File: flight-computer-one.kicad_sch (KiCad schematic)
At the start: 6 parts, among them J3 Screw_Terminal_01x08, J4 Screw_Terminal_01x08

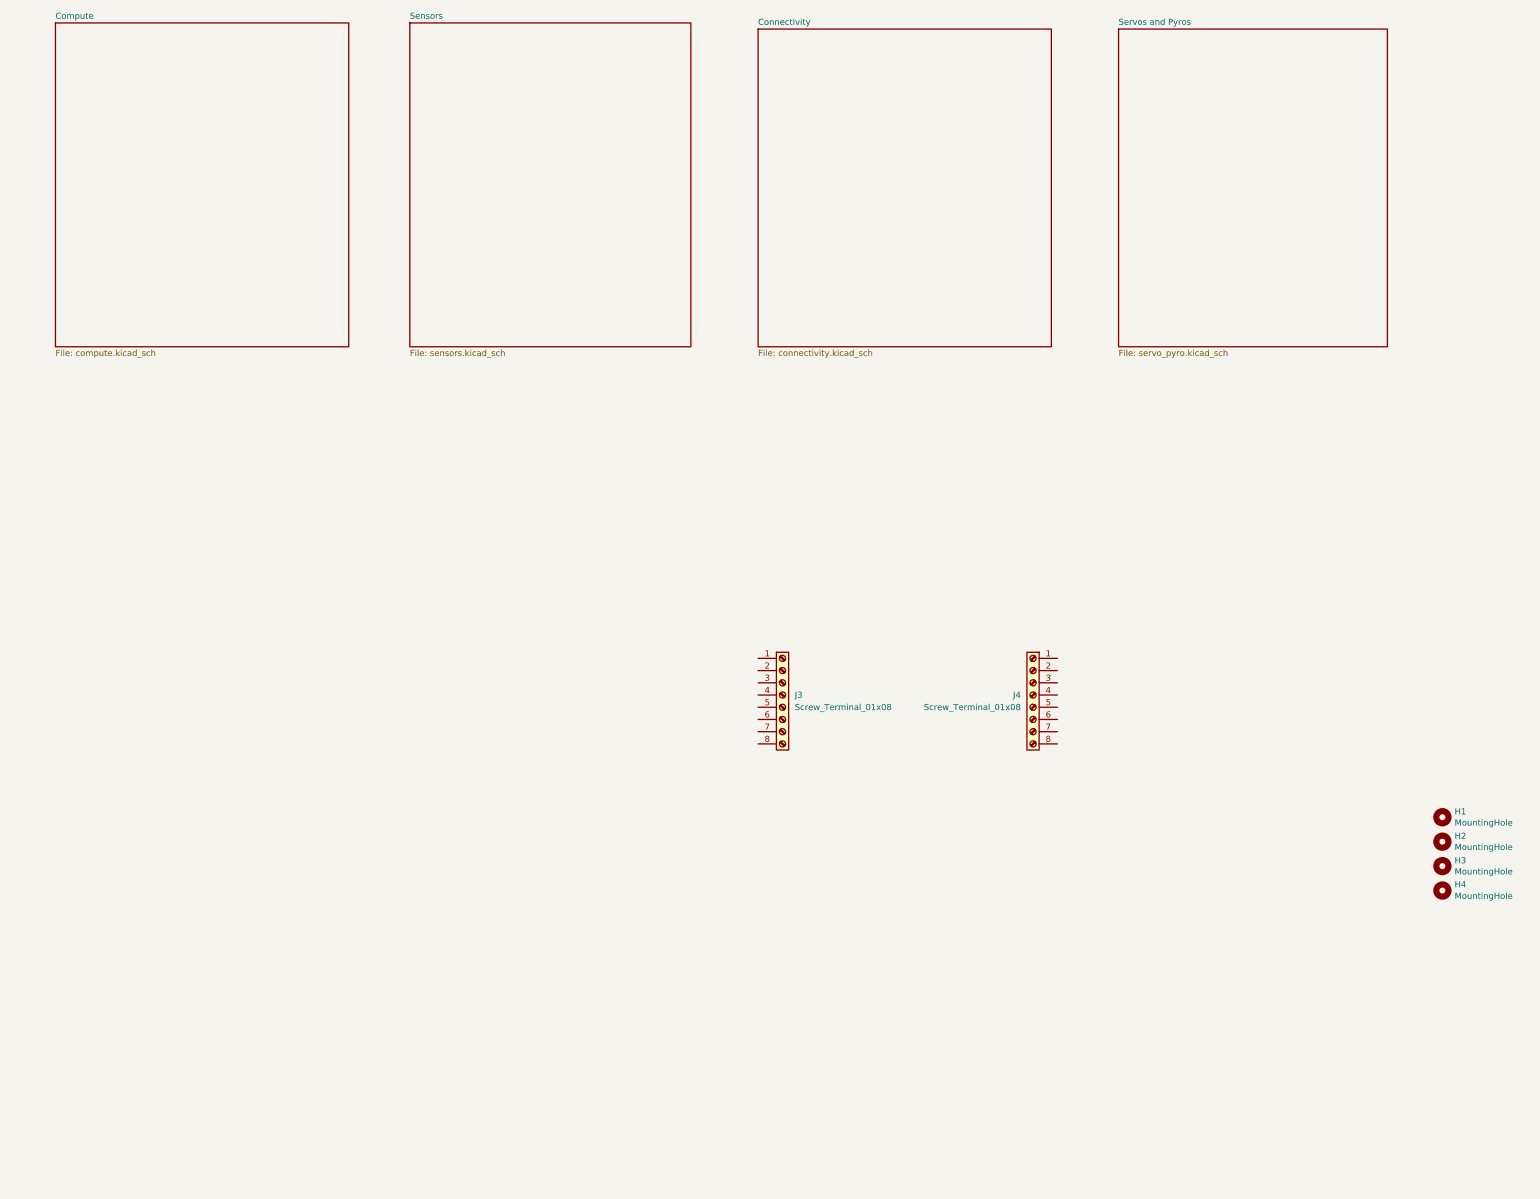
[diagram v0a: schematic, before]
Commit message: created project lib
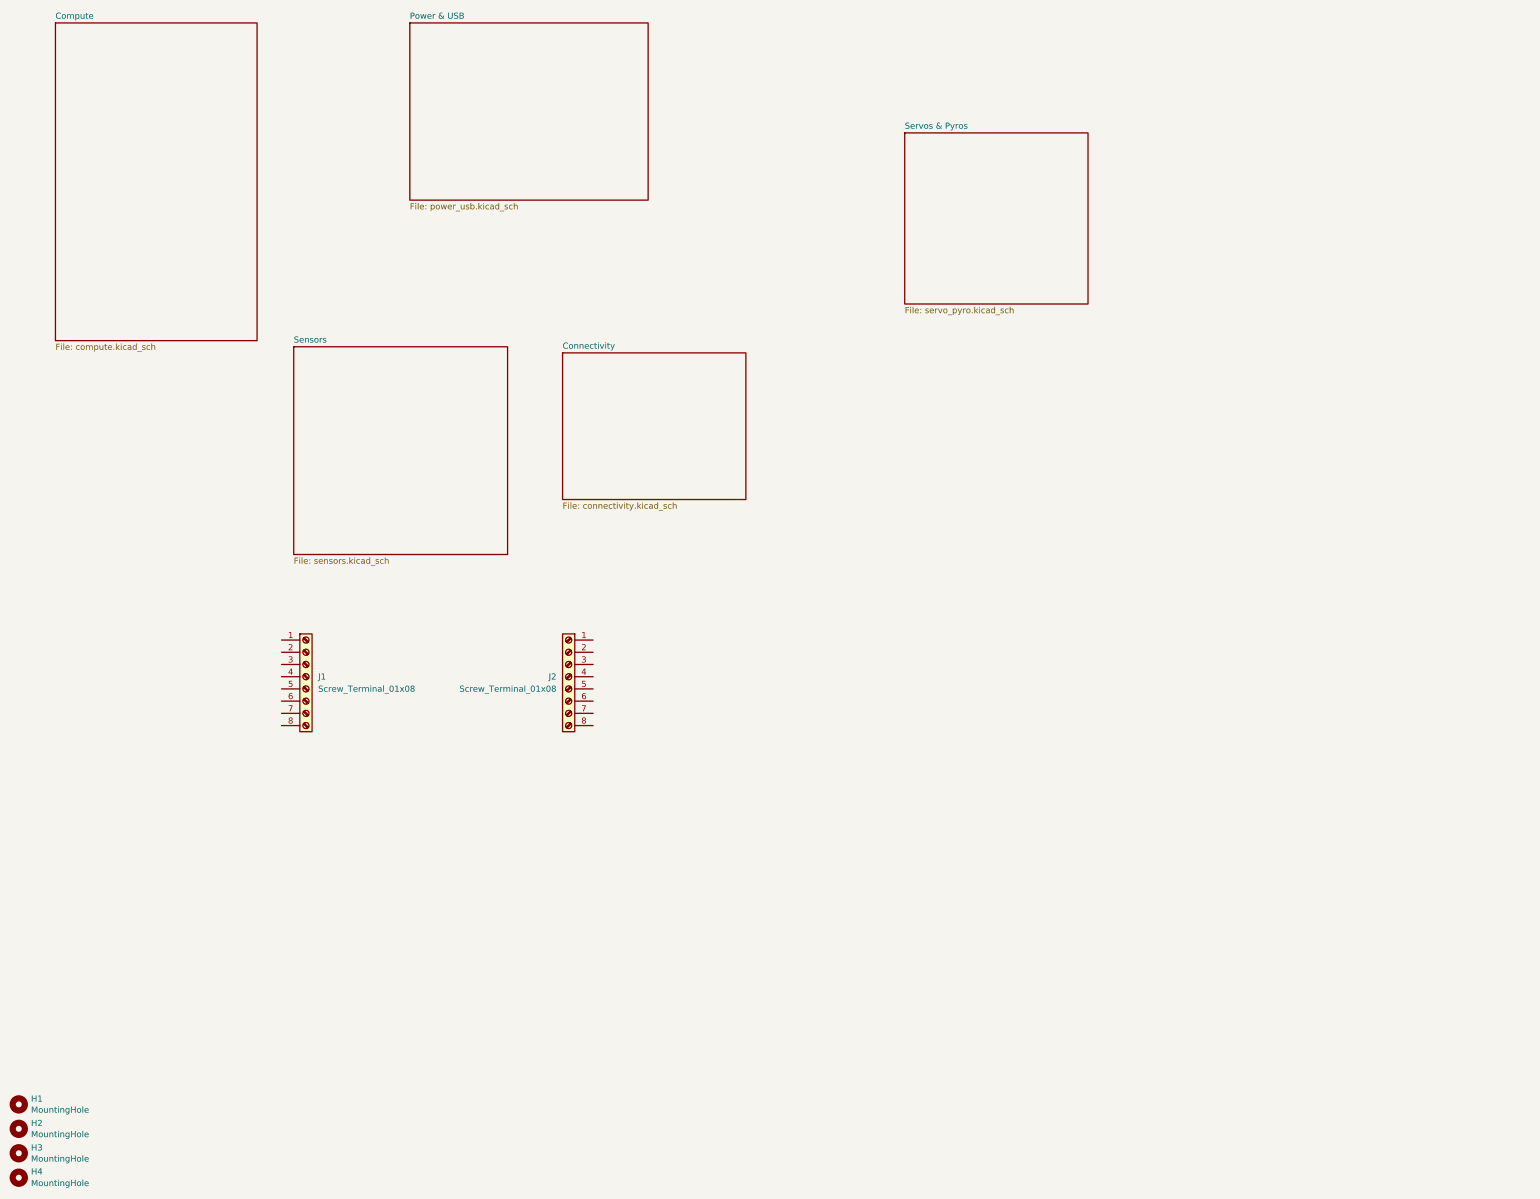
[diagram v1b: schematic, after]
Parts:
- renumbered J3 to J1, J4 to J2
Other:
- sheet Servos and Pyros renamed Servos & Pyros
- added sheet Power & USB (power_usb.kicad_sch)
- moved on the sheet: H1, H2, H3, H4, J1, J2
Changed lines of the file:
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@@
 	(generator "eeschema")
 	(generator_version "9.0")
-	(paper "A3")
+	(paper "A4")
 	(symbol
 		(lib_id "Mechanical:MountingHole")
-		(at 322.58 195.58 0)
+		(at 26.67 255.27 0)
 		(unit 1)
 		(exclude_from_sim no)
@@
 		(dnp no)
 		(property "Reference" "H1"
-			(at 325.12 194.4116 0)
+			(at 29.21 254.1016 0)
 			(effects
 				(font
@@
 		)
 		(property "Value" "MountingHole"
-			(at 325.12 196.723 0)
+			(at 29.21 256.413 0)
 			(effects
 				(font
@@
 		)
 		(property "Footprint" "MountingHole:MountingHole_3.2mm_M3"
-			(at 322.58 195.58 0)
+			(at 26.67 255.27 0)
 			(effects
 				(font
@@
 		)
 		(property "Datasheet" "~"
-			(at 322.58 195.58 0)
+			(at 26.67 255.27 0)
 			(effects
 				(font
@@
 		)
 		(property "Description" ""
-			(at 322.58 195.58 0)
+			(at 26.67 255.27 0)
 			(effects
 				(font
@@
 	(symbol
 		(lib_id "Mechanical:MountingHole")
-		(at 322.58 200.66 0)
+		(at 26.67 260.35 0)
 		(unit 1)
 		(exclude_from_sim no)
@@
 		(dnp no)
 		(property "Reference" "H2"
-			(at 325.12 199.4916 0)
+			(at 29.21 259.1816 0)
 			(effects
 				(font
@@
 		)
 		(property "Value" "MountingHole"
-			(at 325.12 201.803 0)
+			(at 29.21 261.493 0)
 			(effects
 				(font
@@
 		)
 		(property "Footprint" "MountingHole:MountingHole_3.2mm_M3"
-			(at 322.58 200.66 0)
+			(at 26.67 260.35 0)
 			(effects
 				(font
@@
 		)
 		(property "Datasheet" "~"
-			(at 322.58 200.66 0)
+			(at 26.67 260.35 0)
 			(effects
 				(font
@@
 		)
 		(property "Description" ""
-			(at 322.58 200.66 0)
+			(at 26.67 260.35 0)
 			(effects
 				(font
@@
 	(symbol
 		(lib_id "Mechanical:MountingHole")
-		(at 322.58 205.74 0)
+		(at 26.67 265.43 0)
 		(unit 1)
 		(exclude_from_sim no)
@@
 		(dnp no)
 		(property "Reference" "H3"
-			(at 325.12 204.5716 0)
+			(at 29.21 264.2616 0)
 			(effects
 				(font
@@
 		)
 		(property "Value" "MountingHole"
-			(at 325.12 206.883 0)
+			(at 29.21 266.573 0)
 			(effects
 				(font
@@
 		)
 		(property "Footprint" "MountingHole:MountingHole_3.2mm_M3"
-			(at 322.58 205.74 0)
+			(at 26.67 265.43 0)
 			(effects
 				(font
@@
 		)
 		(property "Datasheet" "~"
-			(at 322.58 205.74 0)
+			(at 26.67 265.43 0)
 			(effects
 				(font
@@
 		)
 		(property "Description" ""
-			(at 322.58 205.74 0)
+			(at 26.67 265.43 0)
 			(effects
 				(font
@@
 	(symbol
 		(lib_id "Mechanical:MountingHole")
-		(at 322.58 210.82 0)
+		(at 26.67 270.51 0)
 		(unit 1)
 		(exclude_from_sim no)
@@
 		(dnp no)
 		(property "Reference" "H4"
-			(at 325.12 209.55 0)
+			(at 29.21 269.24 0)
 			(effects
 				(font
@@
 		)
 		(property "Value" "MountingHole"
-			(at 325.12 211.963 0)
+			(at 29.21 271.653 0)
 			(effects
 				(font
@@
 		)
 		(property "Footprint" "MountingHole:MountingHole_3.2mm_M3"
-			(at 322.58 210.82 0)
+			(at 26.67 270.51 0)
 			(effects
 				(font
@@
 		)
 		(property "Datasheet" "~"
-			(at 322.58 210.82 0)
+			(at 26.67 270.51 0)
 			(effects
 				(font
@@
 		)
 		(property "Description" ""
-			(at 322.58 210.82 0)
+			(at 26.67 270.51 0)
 			(effects
 				(font
@@
 	(symbol
 		(lib_id "Connector:Screw_Terminal_01x08")
-		(at 185.42 170.18 0)
+		(at 86.36 166.37 0)
 		(unit 1)
 		(exclude_from_sim no)
@@
 		(dnp no)
 		(fields_autoplaced yes)
-		(property "Reference" "J3"
-			(at 187.96 170.1799 0)
+		(property "Reference" "J1"
+			(at 88.9 166.3699 0)
 			(effects
 				(font
@@
 		)
 		(property "Value" "Screw_Terminal_01x08"
-			(at 187.96 172.7199 0)
+			(at 88.9 168.9099 0)
 			(effects
 				(font
@@
 		)
 		(property "Footprint" "TerminalBlock_Phoenix:TerminalBlock_Phoenix_MKDS-1,5-8_1x08_P5.00mm_Horizontal"
-			(at 185.42 170.18 0)
+			(at 86.36 166.37 0)
 			(effects
 				(font
@@
 		)
 		(property "Datasheet" "~"
-			(at 185.42 170.18 0)
+			(at 86.36 166.37 0)
 			(effects
 				(font
@@
 		)
 		(property "Description" "Generic screw terminal, single row, 01x08, script generated (kicad-library-utils/schlib/autogen/connector/)"
-			(at 185.42 170.18 0)
+			(at 86.36 166.37 0)
 			(effects
 				(font
@@
 			(project ""
 				(path "/2b49a1e7-3a95-411d-8c49-438ba0d49dde"
-					(reference "J3")
+					(reference "J1")
 					(unit 1)
 				)
@@
 	(symbol
 		(lib_id "Connector:Screw_Terminal_01x08")
-		(at 237.49 170.18 0)
+		(at 140.97 166.37 0)
 		(mirror y)
 		(unit 1)
@@
 		(dnp no)
 		(fields_autoplaced yes)
-		(property "Reference" "J4"
-			(at 234.95 170.1799 0)
+		(property "Reference" "J2"
+			(at 138.43 166.3699 0)
 			(effects
 				(font
@@
 		)
 		(property "Value" "Screw_Terminal_01x08"
-			(at 234.95 172.7199 0)
+			(at 138.43 168.9099 0)
 			(effects
 				(font
@@
 		)
 		(property "Footprint" "TerminalBlock_Phoenix:TerminalBlock_Phoenix_MKDS-1,5-8_1x08_P5.00mm_Horizontal"
-			(at 237.49 170.18 0)
+			(at 140.97 166.37 0)
 			(effects
 				(font
@@
 		)
 		(property "Datasheet" "~"
-			(at 237.49 170.18 0)
+			(at 140.97 166.37 0)
 			(effects
 				(font
@@
 		)
 		(property "Description" "Generic screw terminal, single row, 01x08, script generated (kicad-library-utils/schlib/autogen/connector/)"
-			(at 237.49 170.18 0)
+			(at 140.97 166.37 0)
 			(effects
 				(font
@@
 			(project "flight-computer-one"
 				(path "/2b49a1e7-3a95-411d-8c49-438ba0d49dde"
-					(reference "J4")
+					(reference "J2")
 					(unit 1)
 				)
@@
 	(sheet
 		(at 34.29 30.48)
-		(size 60.96 67.31)
+		(size 41.91 66.04)
 		(exclude_from_sim no)
 		(in_bom yes)
@@
 		)
 		(property "Sheetfile" "compute.kicad_sch"
-			(at 34.29 98.3746 0)
+			(at 34.29 97.1046 0)
 			(effects
 				(font
@@
 			(project "flight-computer-one"
 				(path "/2b49a1e7-3a95-411d-8c49-438ba0d49dde"
-					(page "2")
+					(page "3")
 				)
 			)
@@
 	)
 	(sheet
-		(at 180.34 31.75)
-		(size 60.96 66.04)
+		(at 139.7 99.06)
+		(size 38.1 30.48)
 		(exclude_from_sim no)
 		(in_bom yes)
@@
 		)
 		(property "Sheetname" "Connectivity"
-			(at 180.34 31.0384 0)
+			(at 139.7 98.3484 0)
 			(effects
 				(font
@@
 		)
 		(property "Sheetfile" "connectivity.kicad_sch"
-			(at 180.34 98.3746 0)
+			(at 139.7 130.1246 0)
 			(effects
 				(font
@@
 			(project "flight-computer-one"
 				(path "/2b49a1e7-3a95-411d-8c49-438ba0d49dde"
-					(page "4")
+					(page "5")
 				)
 			)
@@
 	)
 	(sheet
-		(at 255.27 31.75)
-		(size 55.88 66.04)
+		(at 107.95 30.48)
+		(size 49.53 36.83)
 		(exclude_from_sim no)
 		(in_bom yes)
@@
 			(color 0 0 0 0.0000)
 		)
-		(property "Sheetname" "Servos and Pyros"
-			(at 255.27 31.0384 0)
+		(property "Sheetname" "Power & USB"
+			(at 107.95 29.7684 0)
 			(effects
 				(font
@@
 			)
 		)
-		(property "Sheetfile" "servo_pyro.kicad_sch"
-			(at 255.27 98.3746 0)
+		(property "Sheetfile" "power_usb.kicad_sch"
+			(at 107.95 67.8946 0)
 			(effects
 				(font
@@
 			(project "flight-computer-one"
 				(path "/2b49a1e7-3a95-411d-8c49-438ba0d49dde"
-					(page "5")
+					(page "2")
 				)
 			)
@@
 	)
 	(sheet
-		(at 107.95 30.48)
-		(size 58.42 67.31)
+		(at 210.82 53.34)
+		(size 38.1 35.56)
 		(exclude_from_sim no)
 		(in_bom yes)
@@
 			(color 0 0 0 0.0000)
 		)
+		(property "Sheetname" "Servos & Pyros"
+			(at 210.82 52.6284 0)
+			(effects
+				(font
+					(size 1.27 1.27)
+				)
+				(justify left bottom)
+			)
+		)
+		(property "Sheetfile" "servo_pyro.kicad_sch"
+			(at 210.82 89.4846 0)
+			(effects
+				(font
+					(size 1.27 1.27)
+				)
+				(justify left top)
+			)
+		)
+		(instances
+			(project "flight-computer-one"
+				(path "/2b49a1e7-3a95-411d-8c49-438ba0d49dde"
+					(page "6")
+				)
+			)
+		)
+	)
+	(sheet
+		(at 83.82 97.79)
+		(size 44.45 43.18)
+		(exclude_from_sim no)
+		(in_bom yes)
+		(on_board yes)
+		(dnp no)
+		(fields_autoplaced yes)
+		(stroke
+			(width 0.1524)
+			(type solid)
+		)
+		(fill
+			(color 0 0 0 0.0000)
+		)
 		(property "Sheetname" "Sensors"
-			(at 107.95 29.7684 0)
+			(at 83.82 97.0784 0)
 			(effects
 				(font
@@
 		)
 		(property "Sheetfile" "sensors.kicad_sch"
-			(at 107.95 98.3746 0)
+			(at 83.82 141.5546 0)
 			(effects
 				(font
@@
 			(project "flight-computer-one"
 				(path "/2b49a1e7-3a95-411d-8c49-438ba0d49dde"
-					(page "3")
-				)
-			)
+					(page "4")
+				)
+			)
